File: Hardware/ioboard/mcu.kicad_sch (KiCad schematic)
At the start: 24 parts, among them U8 STM32F103C8Tx, Y1 8MHz, Y2 32.768K

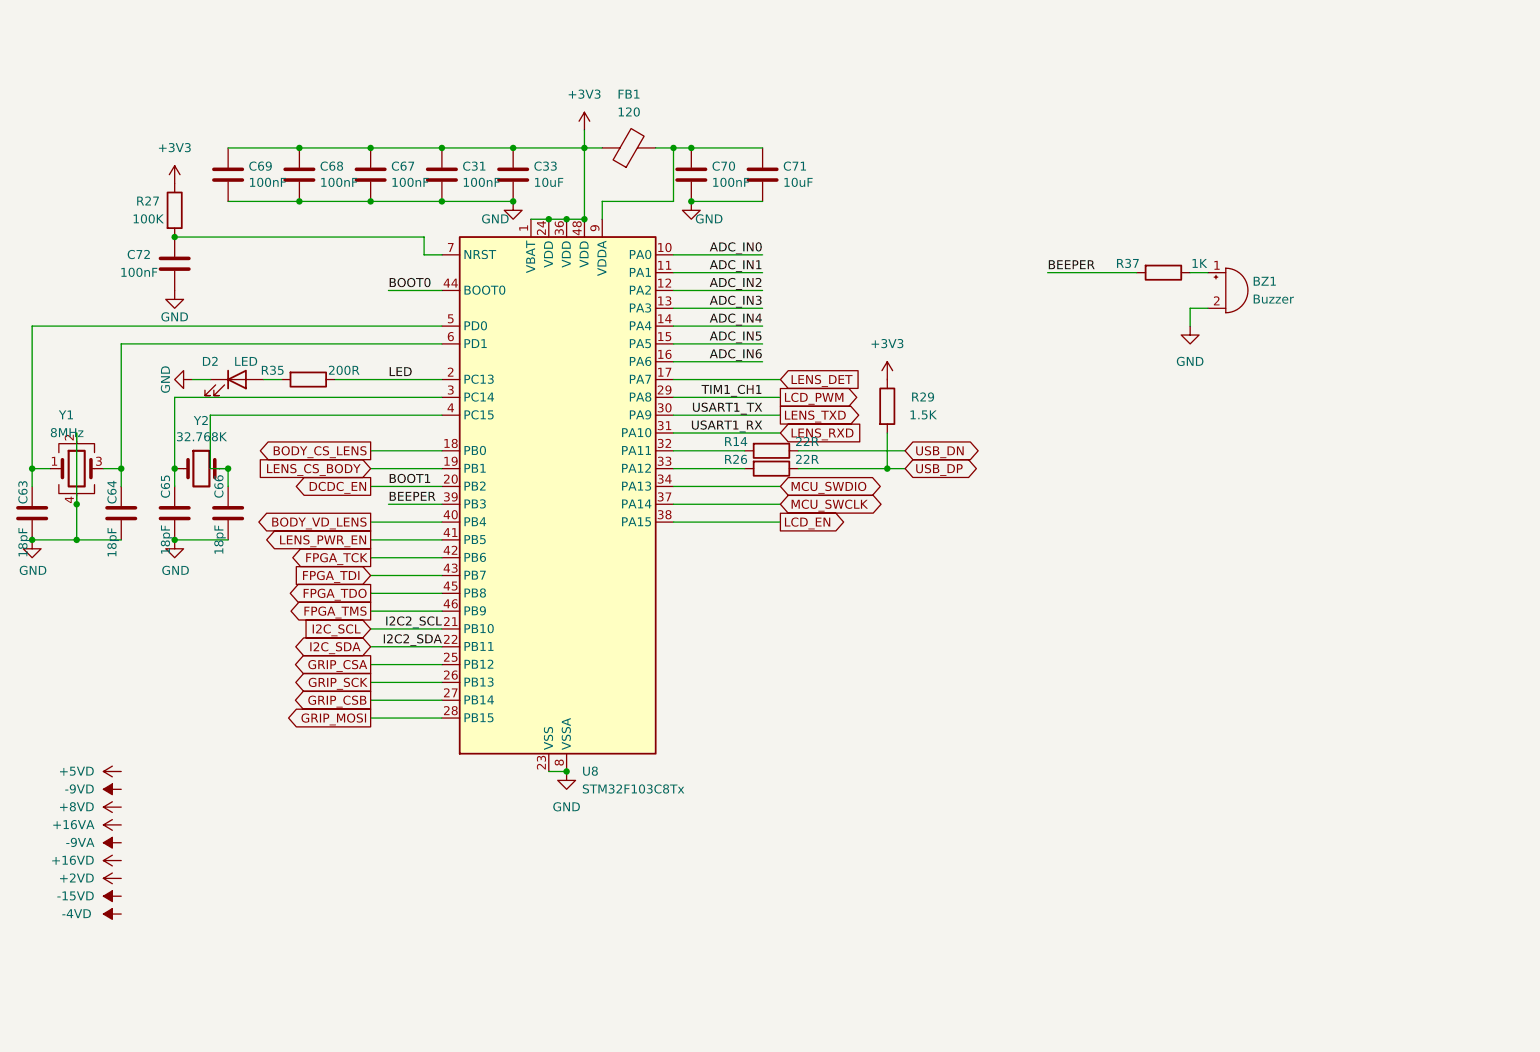
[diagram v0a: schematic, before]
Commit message: Design grip flex, SB/IOB WIP
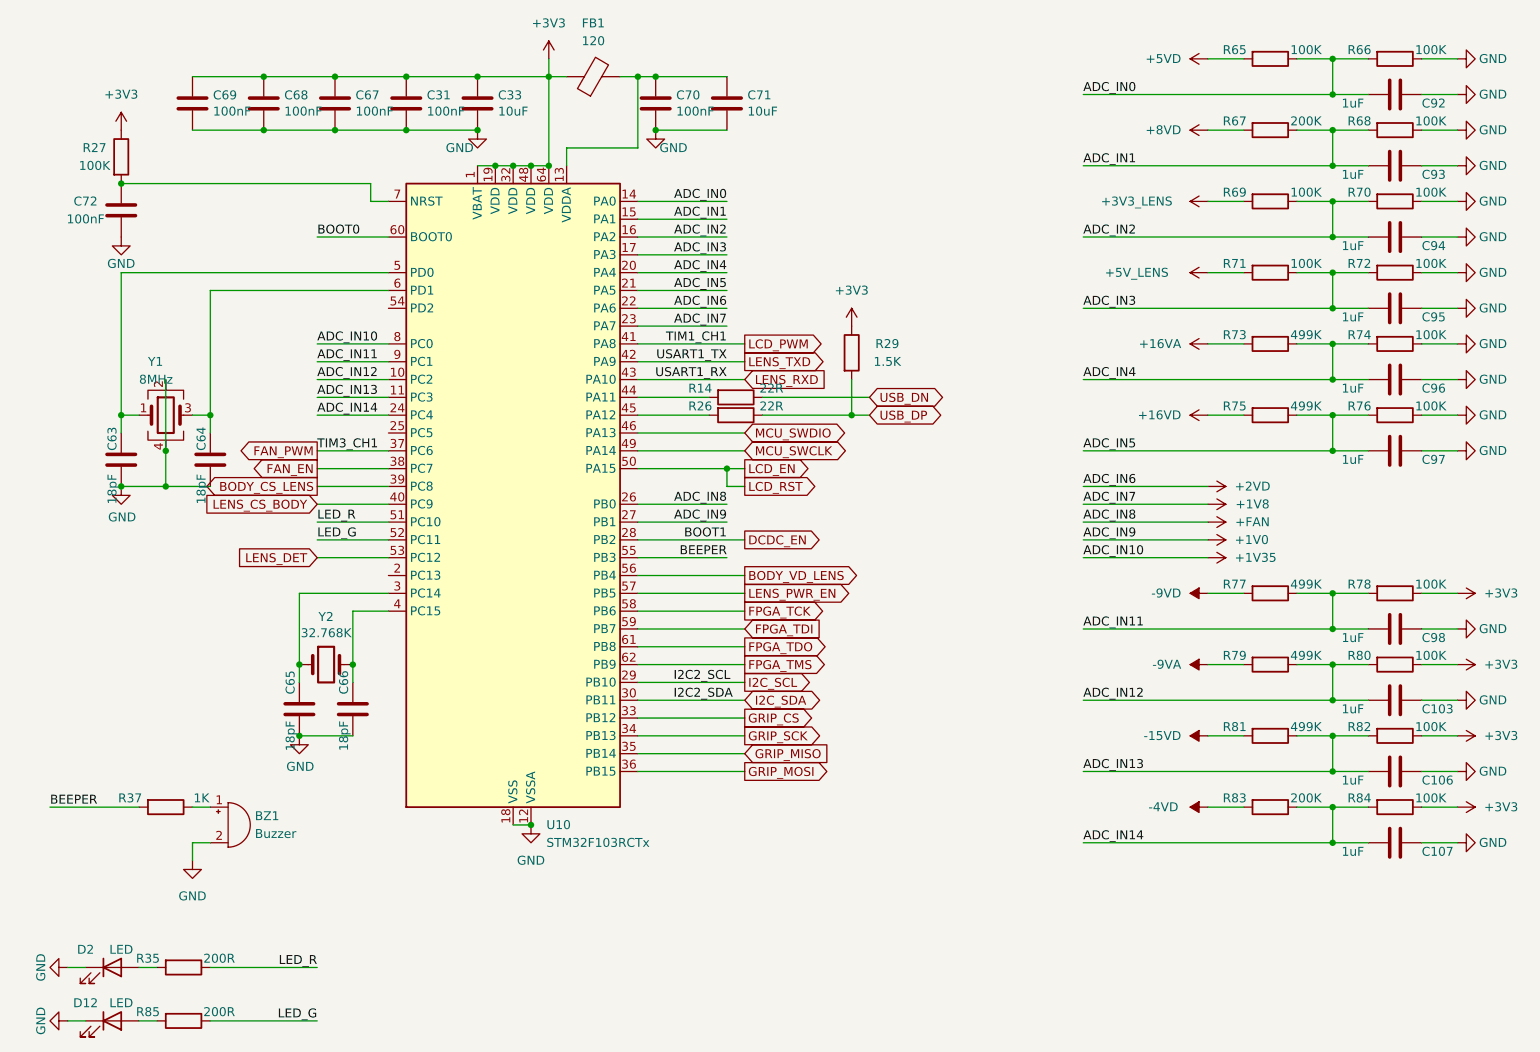
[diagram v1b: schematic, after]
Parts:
- removed U8: STM32F103C8Tx, Package_QFP:LQFP-48_7x7mm_P0.5mm, symbol MCU_ST_STM32F1:STM32F103C8Tx
- added C103, C106, C107, C92, C93, C94, C95, C96, C97, C98: 1uF, Capacitor_SMD:C_0402_1005Metric, symbol Device:C
- added D12: LED, LED_SMD:LED_0603_1608Metric, symbol Device:LED
- added R65, R66, R68, R69, R70, R71, R72, R74, R76, R78, R80, R82, R84: 100K, Resistor_SMD:R_0402_1005Metric, symbol Device:R
- added R67, R83: 200K, Resistor_SMD:R_0402_1005Metric, symbol Device:R
- added R73, R75, R77, R79, R81: 499K, Resistor_SMD:R_0402_1005Metric, symbol Device:R
- added R85: 200R, Resistor_SMD:R_0402_1005Metric, symbol Device:R
- added U10: STM32F103RCTx, Package_QFP:LQFP-64_10x10mm_P0.5mm, symbol MCU_ST_STM32F1:STM32F103RCTx
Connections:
- net +16VA: now also R73.2
- net +16VD: now also R75.2
- net +2VD: now also U10.22 (PA6)
- net +3V3: now also R78.1, R80.1, R82.1, R84.1, U10.1 (VBAT), U10.19 (VDD), U10.32 (VDD), U10.48 (VDD), U10.64 (VDD)
- net +5VD: now also R65.2
- net +8VD: now also R67.2
- net -15VD: now also R81.2
- net -4VD: now also R83.2
- net -9VA: now also R79.2
- net -9VD: now also R77.2
- net ADC_IN0: now also C92.2, R65.1, R66.2, U10.14 (PA0)
- net ADC_IN1: now also C93.2, R67.1, R68.2, U10.15 (PA1)
- net ADC_IN2: now also C94.2, R69.1, R70.2, U10.16 (PA2)
- net ADC_IN3: now also C95.2, R71.1, R72.2, U10.17 (PA3)
- net ADC_IN4: now also C96.2, R73.1, R74.2, U10.20 (PA4)
- net ADC_IN5: now also C97.2, R75.1, R76.2, U10.21 (PA5)
- net BEEPER: now also U10.55 (PB3)
- net BODY_CS_LENS: now also U10.39 (PC8)
- net BODY_VD_LENS: now also U10.56 (PB4)
- net BOOT0: now also U10.60 (BOOT0)
- net DCDC_EN: now also U10.28 (PB2)
- net FPGA_TCK: now also U10.58 (PB6)
- net FPGA_TDI: now also U10.59 (PB7)
- net FPGA_TDO: now also U10.61 (PB8)
- net FPGA_TMS: now also U10.62 (PB9)
- net GND: now also C103.1, C106.1, C107.1, C92.1, C93.1, C94.1, C95.1, C96.1, C97.1, C98.1, D12.1 (K), R66.1, R68.1, R70.1, R72.1, R74.1, R76.1, U10.12 (VSSA), U10.18 (VSS), U10.31 (VSS), U10.47 (VSS), U10.63 (VSS)
- net GRIP_MOSI: now also U10.36 (PB15)
- net GRIP_SCK: now also U10.34 (PB13)
- net I2C_SCL: now also U10.29 (PB10)
- net I2C_SDA: now also U10.30 (PB11)
- net LCD_EN: now also U10.50 (PA15)
- net LCD_PWM: now also U10.41 (PA8)
- net LENS_CS_BODY: now also U10.40 (PC9)
- net LENS_DET: now also U10.53 (PC12)
- net LENS_PWR_EN: now also U10.57 (PB5)
- net LENS_RXD: now also U10.43 (PA10)
- net LENS_TXD: now also U10.42 (PA9)
- net MCU_SWCLK: now also U10.49 (PA14)
- net MCU_SWDIO: now also U10.46 (PA13)
- net at C70.1, C71.1, FB1.2: now also U10.13 (VDDA)
- net at C65.2, Y2.1: now also U10.3 (PC14)
- net at R14.2: now also U10.44 (PA11)
- net at R26.2: now also U10.45 (PA12)
- net at C66.2, Y2.2: now also U10.4 (PC15)
- net at C63.1, Y1.1: now also U10.5 (PD0)
- net at C64.1, Y1.3: now also U10.6 (PD1)
- net at C72.2, R27.2: now also U10.7 (NRST)
- net LED renamed LED_R
- net LED_R: now also U10.51 (PC10)
- new net: D12.2 (A), R85.2
- new net +1V0: U10.27 (PB1)
- new net +1V35: U10.8 (PC0)
- new net +1V8: U10.23 (PA7)
- new net +3V3_LENS: R69.2
- new net +5V_LENS: R71.2
- new net +FAN: U10.26 (PB0)
- new net ADC_IN11: C98.2, R77.1, R78.2, U10.9 (PC1)
- new net ADC_IN12: C103.2, R79.1, R80.2, U10.10 (PC2)
- new net ADC_IN13: C106.2, R81.1, R82.2, U10.11 (PC3)
- new net ADC_IN14: C107.2, R83.1, R84.2, U10.24 (PC4)
- new net FAN_EN: U10.38 (PC7)
- new net FAN_PWM: U10.37 (PC6)
- new net GRIP_CS: U10.33 (PB12)
- new net GRIP_MISO: U10.35 (PB14)
- new net LED_G: R85.1, U10.52 (PC11)
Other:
- moved on the sheet: BZ1, C31, C33, C63, C64, C65, C66, C67, C68, C69, C70, C71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
